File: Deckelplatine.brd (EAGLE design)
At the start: 110 x 75 mm, 57 parts, among them IC1 MAX481CSA, IC2 74HCT595D, IC3 74HCT595D, IC4 74HCT595D, IC5 74HCT595D, IC6 74HCT595D, J1 52808-2570, U1 LM2676S, X1 ''

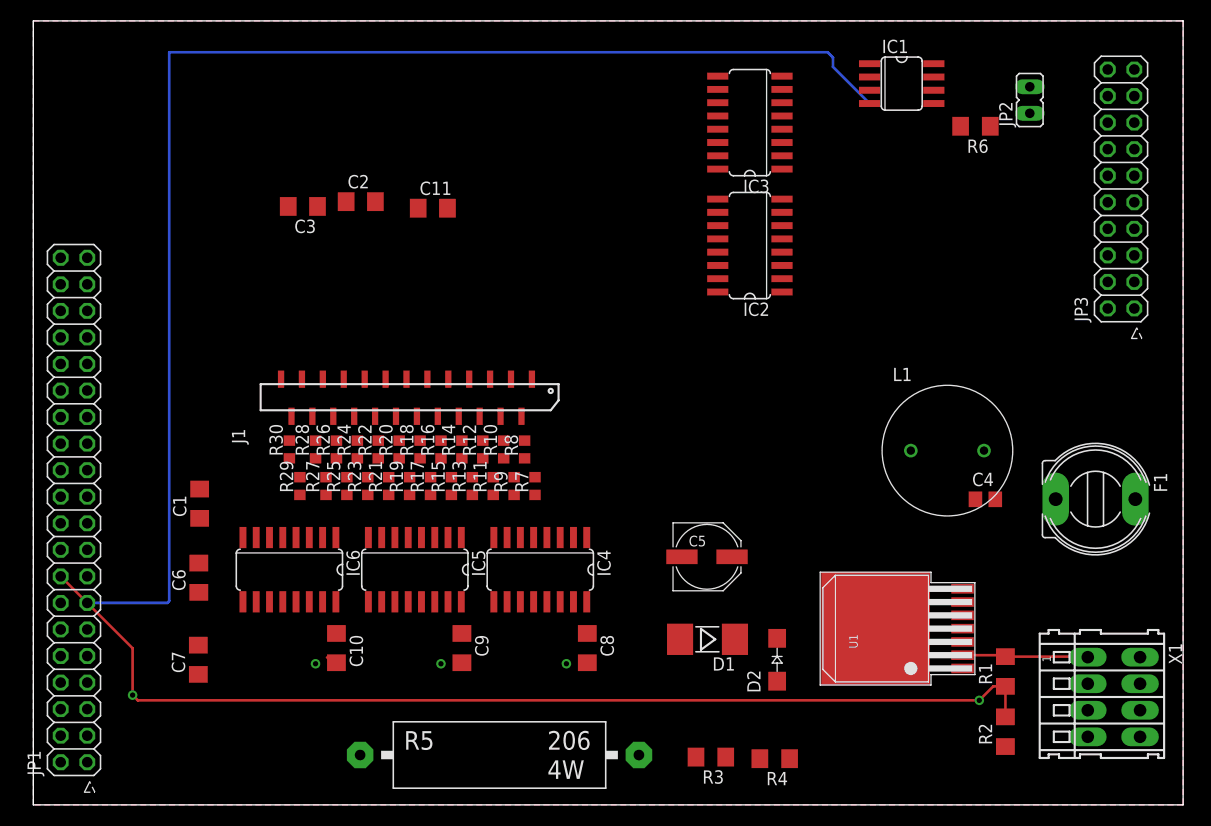
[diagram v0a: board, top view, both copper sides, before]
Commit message: Stromlaufplan fast fertig.
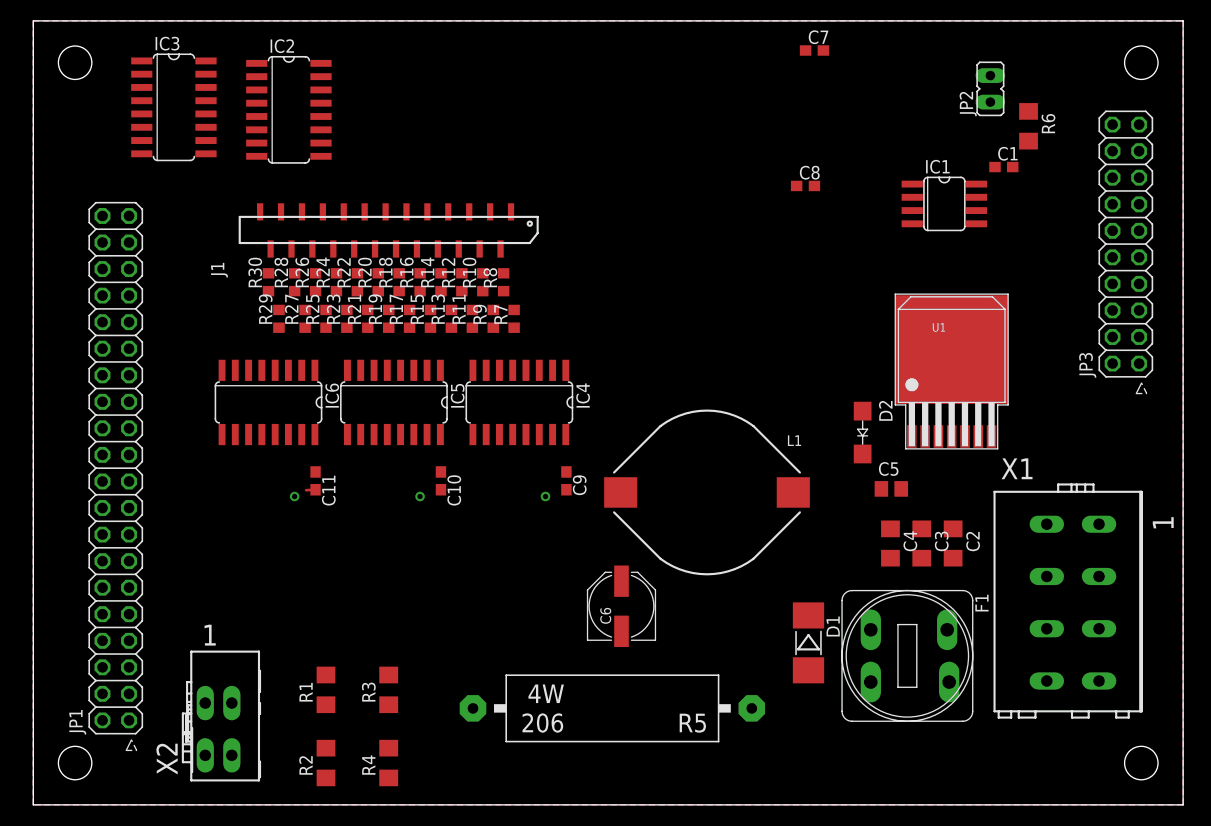
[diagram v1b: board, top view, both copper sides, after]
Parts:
- added X2: 233-502, con-wago_233:P-233-502
- C1, C10, C7, C8, C9: device rcl:C1206 -> resistor:C0603
- C11: value 0.1uF -> 100n; device rcl:C1206 -> resistor:C0603
- C4: value 0.01uF -> 0.1uF; device rcl:C0805 -> rcl:C1206
- C5: value 100uF 16v -> 0.01uF; device rcl:PANASONIC_D -> rcl:C0805
- C6: value 100n -> 100uF 16v; device rcl:C1206 -> rcl:PANASONIC_D
- F1: device fuse:KS9V -> fuse-schurter:3101.0040
- IC1: value MAX481CSA -> MAX1487EESA+
- JP1: value CON6 -> ''
- L1: value 09HCP33UH -> DO5022P-EU_; device Inductor-Fastron:09HCP -> RA-GAS Projekte LTD:DO5022P
- X1: value '' -> 236-404; device con-wago:233-504 -> con-wago_236:P-236-404
- moved C1 83.4 mm to (92.8, 61.0), turned to 0 degrees
- moved C7 82.9 mm to (74.7, 72.2), turned to 0 degrees
- moved C3 67.4 mm to (85.0, 25.0), turned to 270 degrees
- moved C2 65.4 mm to (88.0, 25.0), turned to 270 degrees
- moved R2 65.1 mm to (28.0, 4.00)
- moved R1 65.0 mm to (28.0, 11.0)
- moved IC3 55.1 mm to (13.4, 66.7), turned to 270 degrees
- moved C8 48.9 mm to (73.9, 59.2), turned to 0 degrees
- moved IC2 46.0 mm to (24.4, 66.5), turned to 270 degrees
- moved C6 40.5 mm to (56.3, 19.0)
- moved R4 36.9 mm to (34.0, 4.00), turned to 90 degrees
- moved R3 31.5 mm to (34.0, 11.0), turned to 90 degrees
- moved C11 28.4 mm to (27.0, 31.0), turned to 270 degrees
- moved U1 28.2 mm to (87.9, 44.0), turned to 270 degrees
- moved F1 23.4 mm to (83.6, 14.2)
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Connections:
- net BETRIEB renamed D21
- net BLINK renamed D24
- net N$31 renamed D9
- net N$32 renamed D10
- net N$33 renamed D11
- net N$34 renamed D12
- net N$35 renamed D13
- net N$36 renamed D14
- net N$37 renamed D15
- net N$38 renamed D16
- net STOERUNG renamed D22
- net WARTUNG renamed D23
- new net N$31: F1.3, F1.4
- net 12V_VIN: now also C4.1, X1.L1.1, X1.L1.2; no longer C11.1, X1.B1
- net ACCU+: now also F1.2, X1.L3.1, X1.L3.2; no longer X1.B3
- net ACCU-: now also X1.L4.1, X1.L4.2; no longer X1.B4
- net GND: now also C4.2, C6.-, X1.L2.1, X1.L2.2, X2.L2.1, X2.L2.2; no longer C5.-, C6.2, X1.B2
- net N$1: no longer F1.2
- net N$42: now also C5.2; no longer C4.2
- net N$44: now also C5.1, L1.1; no longer C4.1, L1.P$2
- net VCC: now also C11.1, C6.+, L1.2, X2.L1.1, X2.L1.2; no longer C5.+, C6.1, L1.P$1
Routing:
- net TXD: track 130.1 -> 0.00 mm
- net MON_MAINS: track 101.4 -> 0.00 mm
- net 12V_VIN: track 12.4 -> 0.00 mm
- net VCC: track 0.56 -> 0.00 mm
